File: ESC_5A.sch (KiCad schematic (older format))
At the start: 23 parts, among them IC1 EEPROM, IC2 3.3V Reg, IC3 5V_Reg, IC4 ATSAMD21E17D-AUT, J1 USBc, J2 5V_PWR

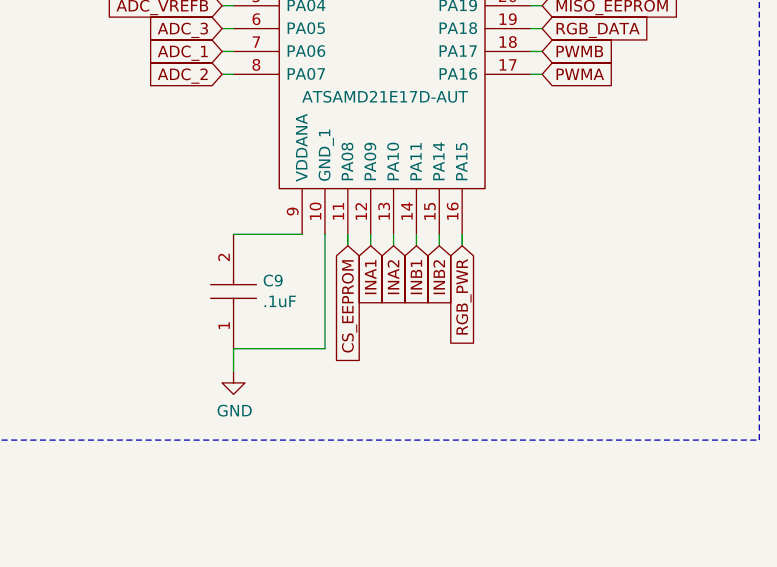
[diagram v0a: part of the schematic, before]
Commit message: testing other options
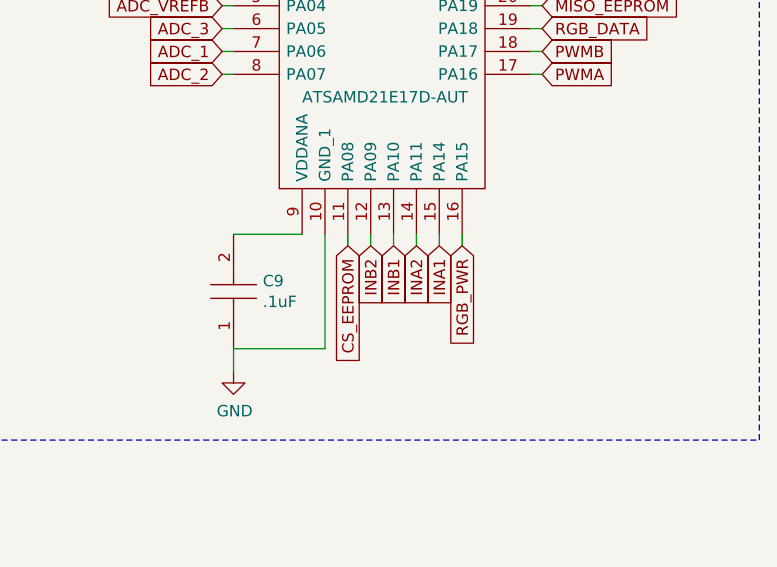
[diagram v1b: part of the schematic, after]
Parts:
- L1: footprint SamacSys_Parts:INDM8680X300N -> SamacSys_Parts:XAL6060333MEC
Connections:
- net INA1: now also IC4.15 (PA14); no longer IC4.12 (PA09)
- net INA2: now also IC4.14 (PA11); no longer IC4.13 (PA10)
- net INB1: now also IC4.13 (PA10); no longer IC4.14 (PA11)
- net INB2: now also IC4.12 (PA09); no longer IC4.15 (PA14)
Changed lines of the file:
@@
 Text GLabel 10100 4750 2    50   Input ~ 0
 PWMB
+Text GLabel 9450 5600 3    50   Input ~ 0
+INB1
+Text GLabel 9350 5600 3    50   Input ~ 0
+INB2
+Text GLabel 9650 5600 3    50   Input ~ 0
+INA1
 Text GLabel 9550 5600 3    50   Input ~ 0
-INB1
-Text GLabel 9650 5600 3    50   Input ~ 0
-INB2
-Text GLabel 9350 5600 3    50   Input ~ 0
-INA1
-Text GLabel 9450 5600 3    50   Input ~ 0
 INA2
 Text GLabel 9750 3300 1    50   Input ~ 0
@@
 F 0 "L1" H 5350 5675 50  0000 C CNN
 F 1 "33uH" H 5350 5584 50  0000 C CNN
-F 2 "SamacSys_Parts:INDM8680X300N" H 5600 5500 50  0001 L CNN
+F 2 "SamacSys_Parts:XAL6060333MEC" H 5600 5500 50  0001 L CNN
 F 3 "https://componentsearchengine.com/Datasheets/1/MPX1D0830L330.pdf" H 5600 5400 50  0001 L CNN
 F 4 "Metal Composite Power Inductors MPX" H 5600 5300 50  0001 L CNN "Description"
